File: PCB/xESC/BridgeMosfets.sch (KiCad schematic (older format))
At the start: 6 parts, among them Q1 BSC440N10NS3G, Q2 BSC440N10NS3G

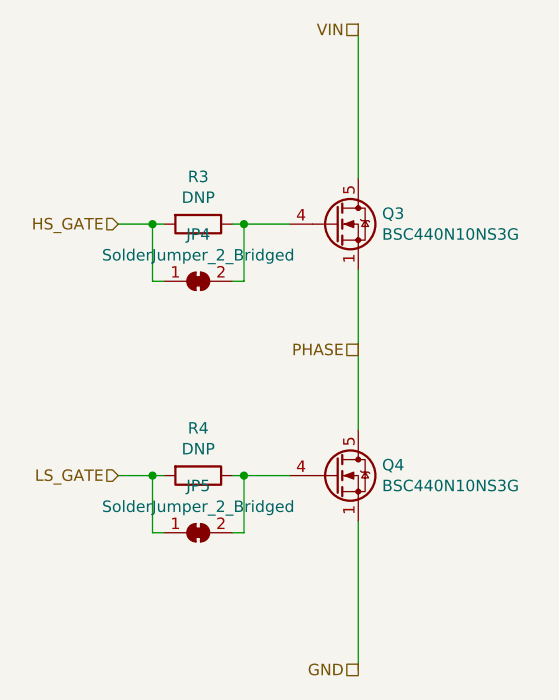
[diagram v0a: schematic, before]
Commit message: wip
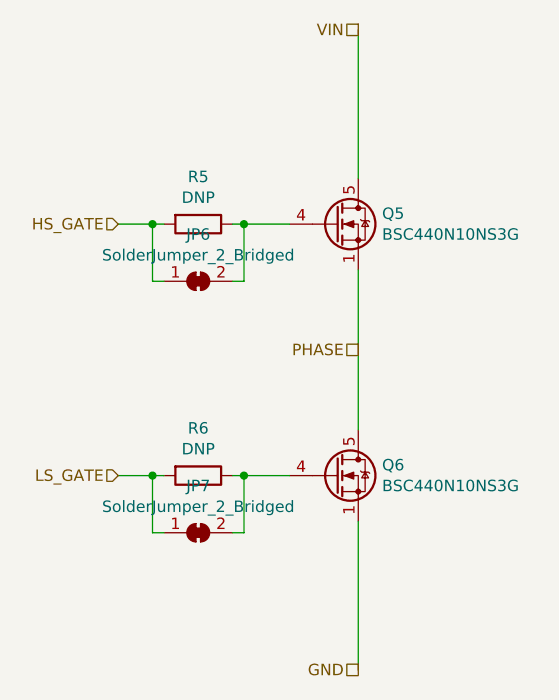
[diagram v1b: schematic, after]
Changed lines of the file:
@@
 $Descr A4 11693 8268
 encoding utf-8
-Sheet 5 6
+Sheet 6 6
 Title "xESC BLDC Controller"
 Date "2021-11-02"
@@
 AR Path="/6183112C/618D9FC1/618746CC" Ref="Q3"  Part="1"
 AR Path="/6183112C/618DC168/618746CC" Ref="Q5"  Part="1"
-F 0 "Q3" H 3704 2396 50  0000 L CNN
+F 0 "Q5" H 3704 2396 50  0000 L CNN
 F 1 "BSC440N10NS3G" H 3704 2305 50  0000 L CNN
 F 2 "Package_TO_SOT_SMD:TDSON-8-1" H 3700 2275 50  0001 L CIN
@@
 AR Path="/6183112C/618D9FC1/6187B610" Ref="Q4"  Part="1"
 AR Path="/6183112C/618DC168/6187B610" Ref="Q6"  Part="1"
-F 0 "Q4" H 3704 3496 50  0000 L CNN
+F 0 "Q6" H 3704 3496 50  0000 L CNN
 F 1 "BSC440N10NS3G" H 3704 3405 50  0000 L CNN
 F 2 "Package_TO_SOT_SMD:TDSON-8-1" H 3700 3375 50  0001 L CIN
@@
 AR Path="/6183112C/618D9FC1/619384E2" Ref="R3"  Part="1"
 AR Path="/6183112C/618DC168/619384E2" Ref="R5"  Part="1"
-F 0 "R3" V 2693 2350 50  0000 C CNN
+F 0 "R5" V 2693 2350 50  0000 C CNN
 F 1 "DNP" V 2784 2350 50  0000 C CNN
 F 2 "Resistor_SMD:R_0805_2012Metric" V 2830 2350 50  0001 C CNN
@@
 AR Path="/6183112C/618D9FC1/6193ABD6" Ref="R4"  Part="1"
 AR Path="/6183112C/618DC168/6193ABD6" Ref="R6"  Part="1"
-F 0 "R4" V 2693 3450 50  0000 C CNN
+F 0 "R6" V 2693 3450 50  0000 C CNN
 F 1 "DNP" V 2784 3450 50  0000 C CNN
 F 2 "Resistor_SMD:R_0805_2012Metric" V 2830 3450 50  0001 C CNN
@@
 AR Path="/6183112C/618D9FC1/6193ADCE" Ref="JP4"  Part="1"
 AR Path="/6183112C/618DC168/6193ADCE" Ref="JP6"  Part="1"
-F 0 "JP4" H 2900 2805 50  0000 C CNN
+F 0 "JP6" H 2900 2805 50  0000 C CNN
 F 1 "SolderJumper_2_Bridged" H 2900 2714 50  0000 C CNN
 F 2 "Jumper:SolderJumper-2_P1.3mm_Bridged_Pad1.0x1.5mm" H 2900 2600 50  0001 C CNN
@@
 AR Path="/6183112C/618D9FC1/6193C72B" Ref="JP5"  Part="1"
 AR Path="/6183112C/618DC168/6193C72B" Ref="JP7"  Part="1"
-F 0 "JP5" H 2900 3905 50  0000 C CNN
+F 0 "JP7" H 2900 3905 50  0000 C CNN
 F 1 "SolderJumper_2_Bridged" H 2900 3814 50  0000 C CNN
 F 2 "Jumper:SolderJumper-2_P1.3mm_Bridged_Pad1.0x1.5mm" H 2900 3700 50  0001 C CNN
